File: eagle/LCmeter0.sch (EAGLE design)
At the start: 25 parts, among them IC1 PIC16F876A-X/SP, K2 DS2Y, Q1 20MHz, Q2 BC548, SW1 SPST, SW2 DPDT

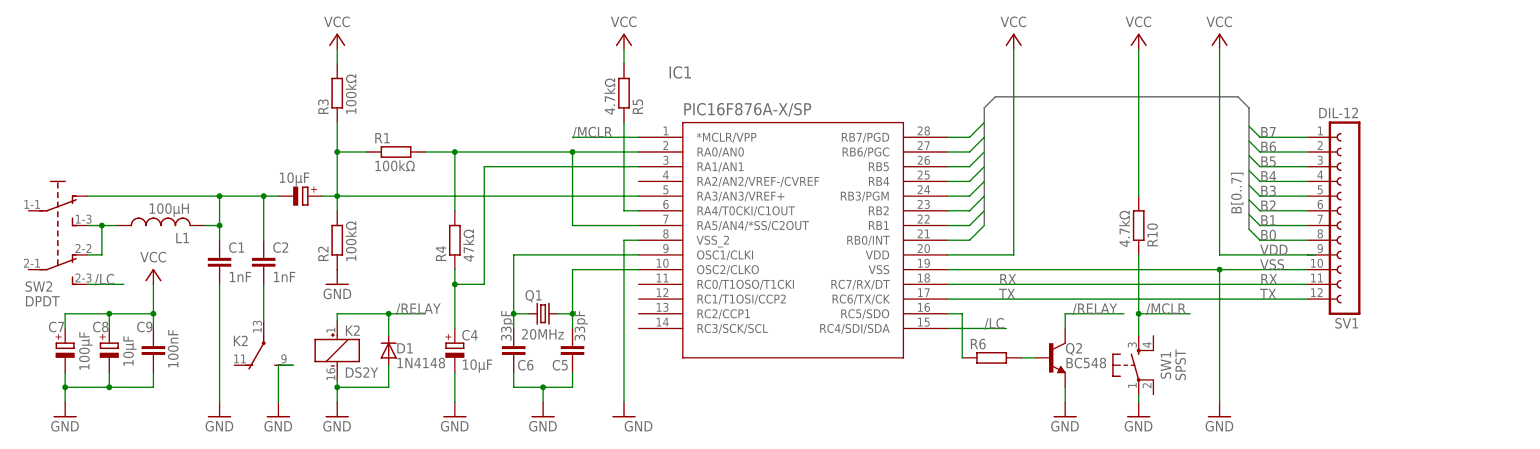
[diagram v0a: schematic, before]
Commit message: ...
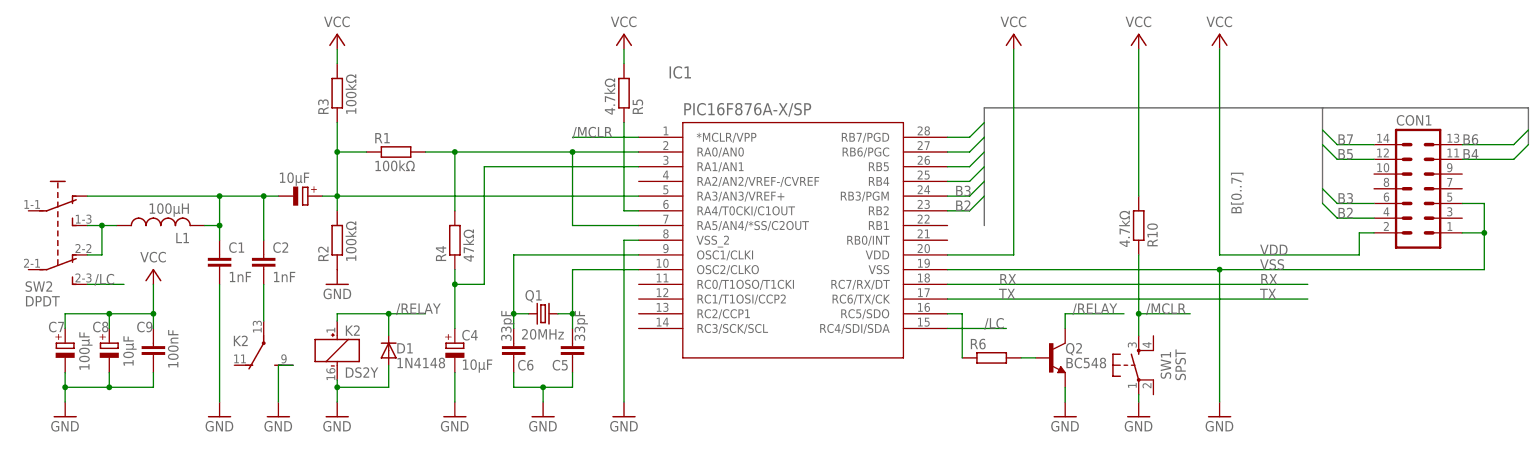
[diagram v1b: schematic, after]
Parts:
- removed SV1: DIL-12, con-lsta:FE12-1
- added CON1: (no value), con-lstb:MA07-2
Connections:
- removed net B0: IC1.RB0/INT, SV1.8
- removed net B1: IC1.RB1, SV1.7
- net B2: now also CON1.4; no longer SV1.6
- net B3: now also CON1.6; no longer SV1.5
- net B4: now also CON1.11; no longer SV1.4
- net B5: now also CON1.12; no longer SV1.3
- net B6: now also CON1.13; no longer SV1.2
- net B7: now also CON1.14; no longer SV1.1
- net N$3: now also CON1.2; no longer SV1.9
- net RX: no longer SV1.11
- net TX: no longer SV1.12
- net VSS: now also CON1.1, CON1.5; no longer SV1.10
